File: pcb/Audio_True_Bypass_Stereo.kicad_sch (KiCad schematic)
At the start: 12 parts, among them J2 AUDIO_IN_TRS, J4 AUDIO_OUT_TRS, K1 G6K-2, K2 G6K-2, Q1 SS8050, U5 CPC1018N, U6 CPC1018N

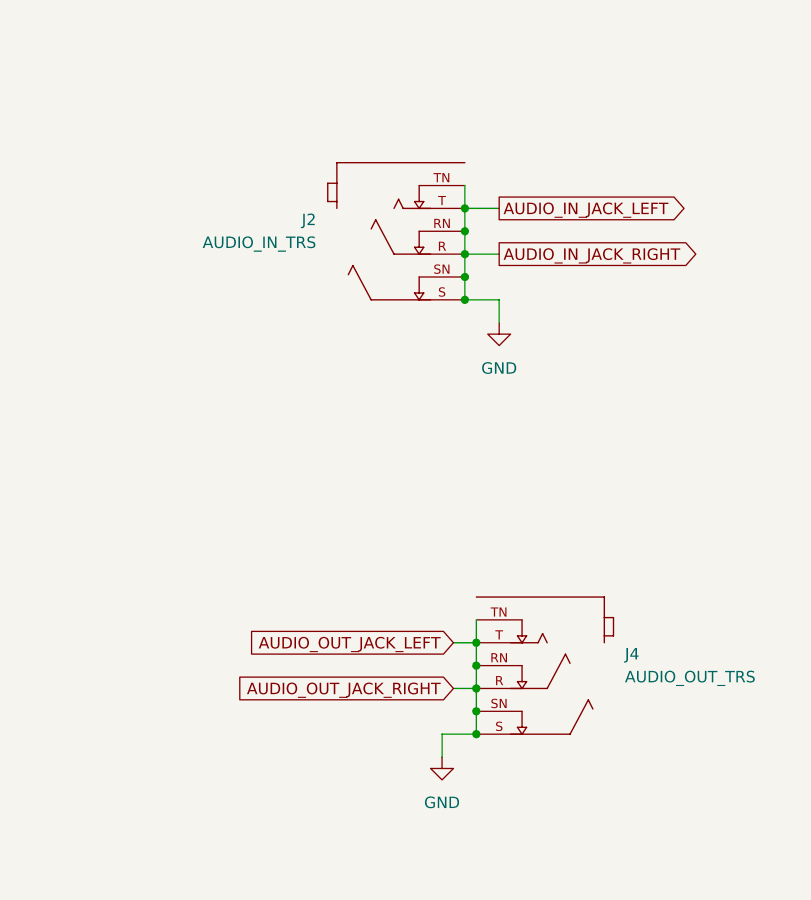
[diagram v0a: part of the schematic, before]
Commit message: Updated kiCad FIles
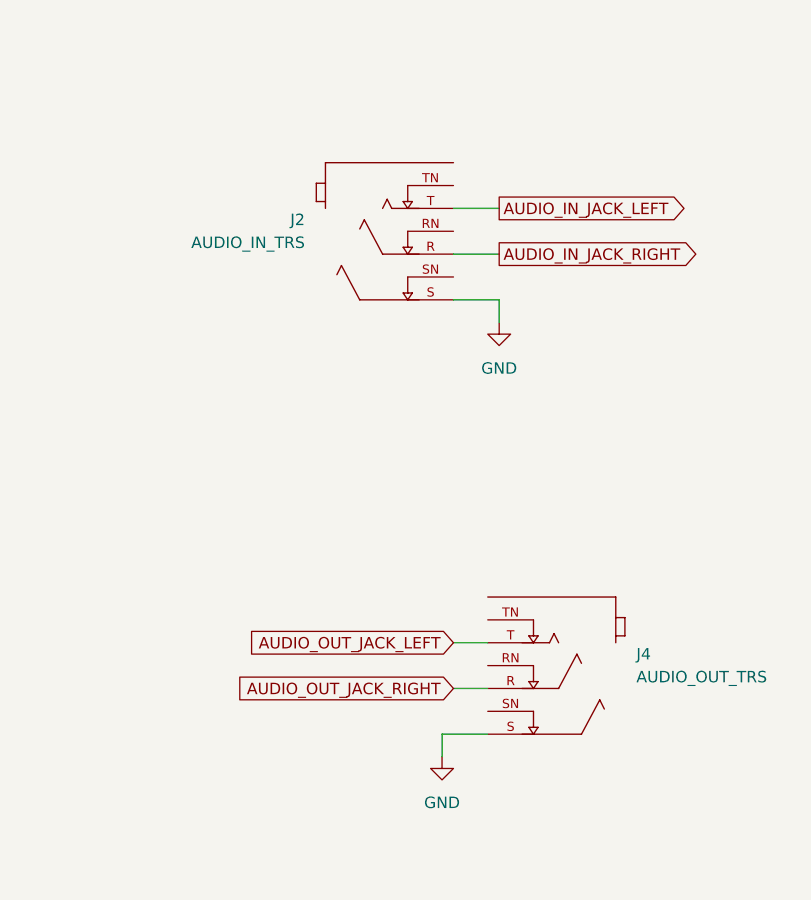
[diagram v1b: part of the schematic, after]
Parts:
- J2, J4: footprint NMJ6HCD2:NEUTRIK_NMJ6HCD2 -> Connector_Audio:Jack_6.35mm_Neutrik_NMJ6HCD2_Horizontal
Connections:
- net GND: no longer J2.R, J2.RN, J2.SN, J2.T, J2.TN, J4.R, J4.RN, J4.SN, J4.T, J4.TN, K1.4, K1.6, K1.7, K2.4, K2.6, K2.7, U5.4, U6.4
- new net AUDIO_IN_JACK_LEFT: J2.T, K1.4, K1.7
- new net AUDIO_IN_JACK_RIGHT: J2.R, K2.4, K2.7
- new net AUDIO_OUT_JACK_LEFT: J4.T, K1.6, U5.4
- new net AUDIO_OUT_JACK_RIGHT: J4.R, K2.6, U6.4
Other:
- moved on the sheet: J2, J4
